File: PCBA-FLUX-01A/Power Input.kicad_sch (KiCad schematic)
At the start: 31 parts, among them Q1 IPT015N10N5, U1 LM74700

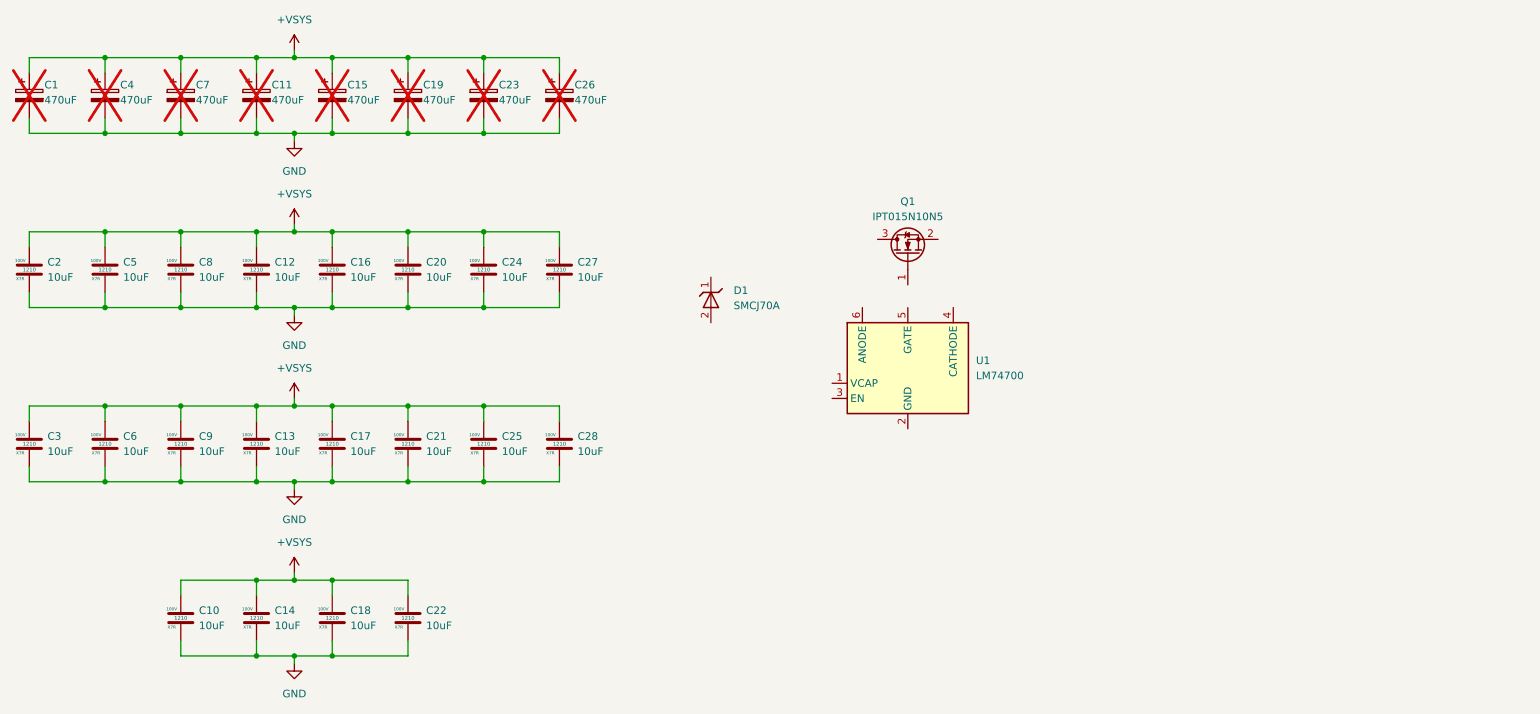
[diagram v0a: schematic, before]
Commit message: Changes were made
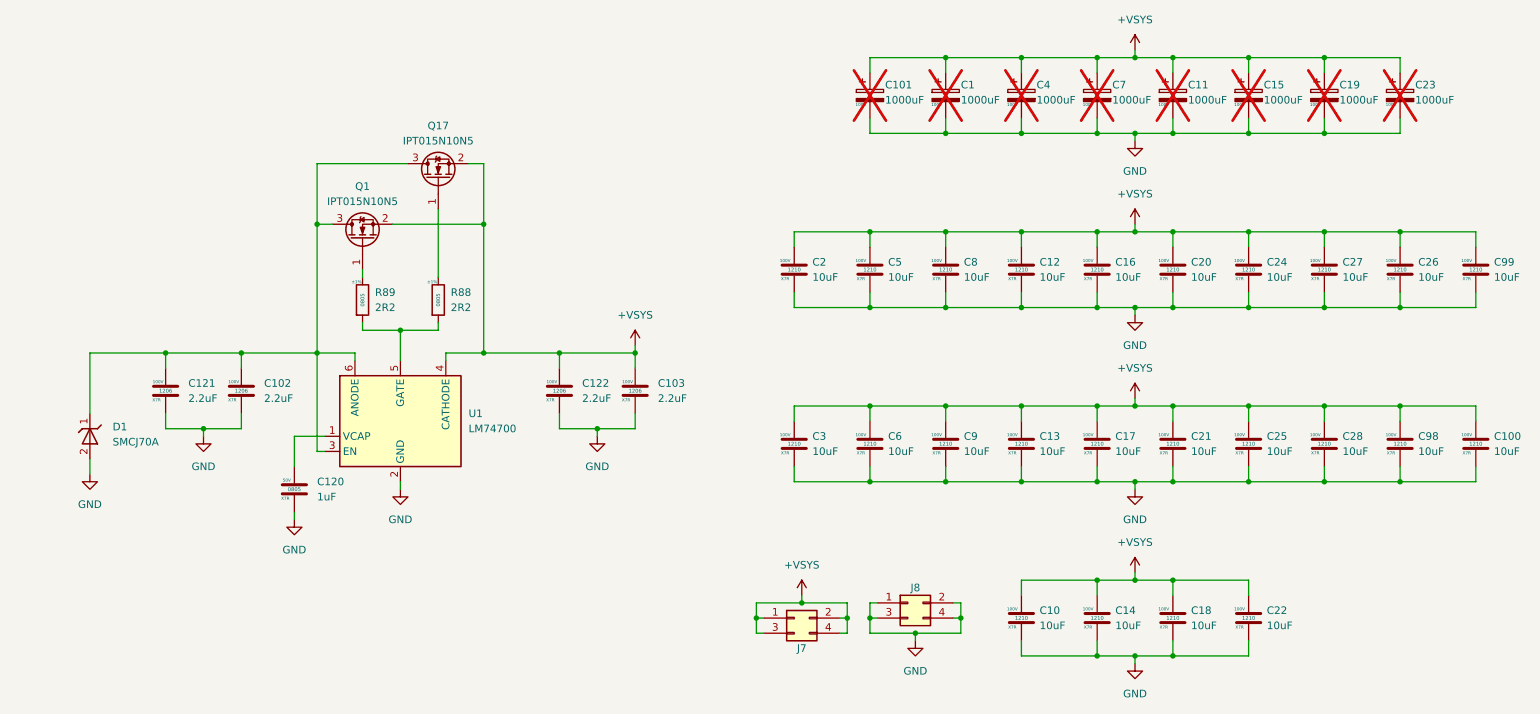
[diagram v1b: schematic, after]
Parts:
- removed C26: 470uF, Capacitor_THT:CP_Radial_D17.0mm_P7.50mm, symbol Device:C_Polarized
- added C100, C26, C98, C99: 10uF, Capacitor_SMD:C_1210_3225Metric, symbol Device:C
- added C101: 1000uF, Capacitor_THT:CP_Radial_D18.0mm_P7.50mm, symbol Device:C_Polarized
- added C102, C103, C121, C122: 2.2uF, Capacitor_SMD:C_1206_3216Metric, symbol Device:C
- added C120: 1uF, Capacitor_SMD:C_0805_2012Metric, symbol Device:C
- added J7, J8: Conn_02x02_Odd_Even, Connector_PinHeader_2.54mm:PinHeader_2x02_P2.54mm_Vertical, symbol Connector_Generic:Conn_02x02_Odd_Even
- added Q17: IPT015N10N5, Package_TO_SOT_SMD:Infineon_PG-HSOF-8-1_ThermalVias, symbol Bvrny's_library:IPT015N10N5
- added R88, R89: 2R2, Resistor_SMD:R_0805_2012Metric, symbol Device:R
- C1, C11, C15, C19, C23, C4, C7: value 470uF -> 1000uF; footprint Capacitor_THT:CP_Radial_D17.0mm_P7.50mm -> Capacitor_THT:CP_Radial_D18.0mm_P7.50mm
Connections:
- net +VSYS: now also Q1.2, U1.4 (CATHODE), C100.1, C101.1, C103.1, C122.1, C26.1, C98.1, C99.1, J7.1 (Pin_1), J7.2 (Pin_2), J7.3 (Pin_3), J7.4 (Pin_4), Q17.2
- net GND: now also D1.2, U1.2 (GND), C100.2, C101.2, C102.2, C103.2, C120.2, C121.2, C122.2, C26.2, C98.2, C99.2, J8.1 (Pin_1), J8.2 (Pin_2), J8.3 (Pin_3), J8.4 (Pin_4)
- net at D1.1: now also Q1.3, U1.3 (EN), U1.6 (ANODE), C102.1, C121.1, Q17.3
- net at Q1.1: now also R89.1
- net at U1.1 (VCAP): now also C120.1
- net at U1.5 (GATE): now also R88.2, R89.2
- new net: Q17.1, R88.1
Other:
- moved on the sheet: C1, C10, C12, C13, C14, C16, C17, C18, C2, C20, C21, C22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
